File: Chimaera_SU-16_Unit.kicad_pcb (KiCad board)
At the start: 2 copper layers, 80 x 30 mm, 66 parts, among them P0 CONN_4, P1 CONN_4, P2 CONN_3, U0 CD74HC4067, U1 MCP602, U2 MCP1703

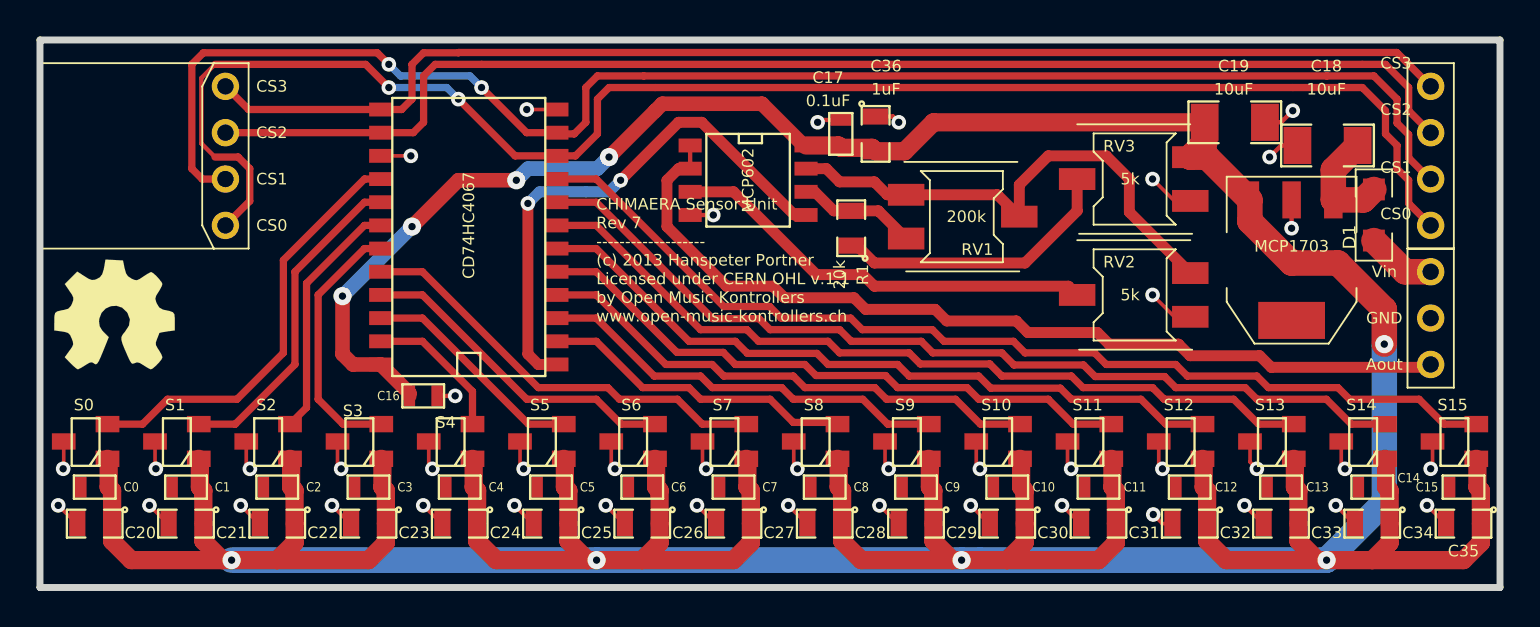
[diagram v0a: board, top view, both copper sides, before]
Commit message: last changes for Alpha Batch PCBs
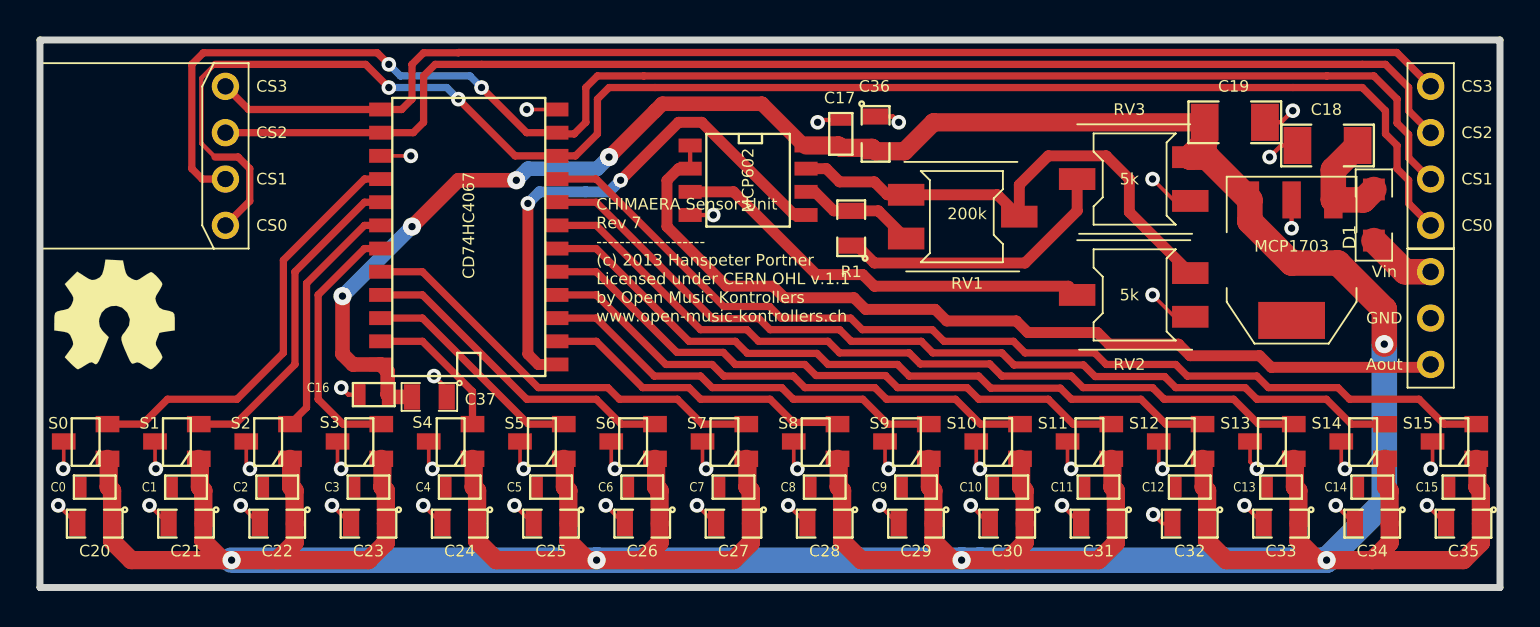
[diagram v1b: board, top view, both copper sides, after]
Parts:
- added C37: 1uF, SM0805, F.Cu at (33.3, 31.6)
- moved C16 2.71 mm to (30.3, 31.4), turned to 0 degrees
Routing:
- net GND: track 66.9 -> 68.6 mm, vias 43 -> 44
- net Vcc: track 302.4 -> 303.2 mm
